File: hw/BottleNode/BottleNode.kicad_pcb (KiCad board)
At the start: 2 copper layers, 29 x 40 mm, 16 parts, among them J1 Conn_01x03_Pin, J2 Conn_01x02_Pin

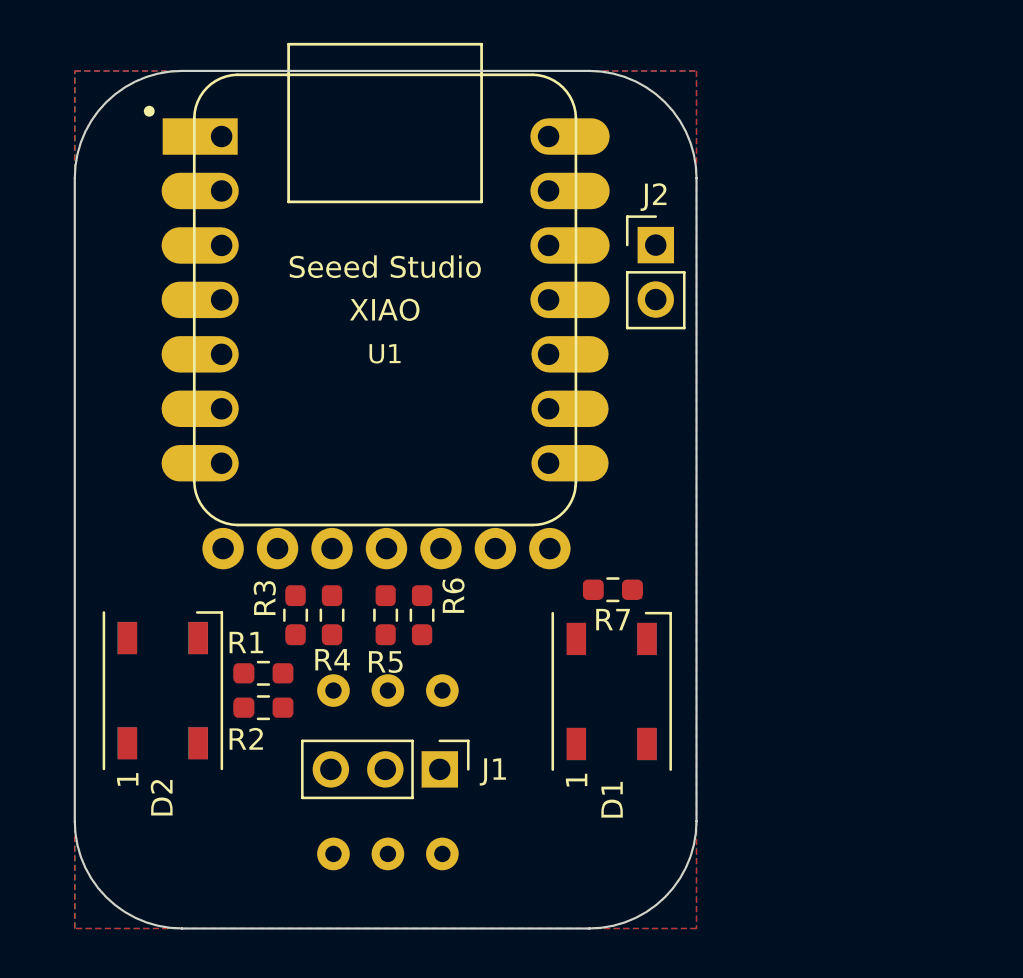
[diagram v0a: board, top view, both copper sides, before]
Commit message: rev 1.1 of schematic and PCB layout with BOM
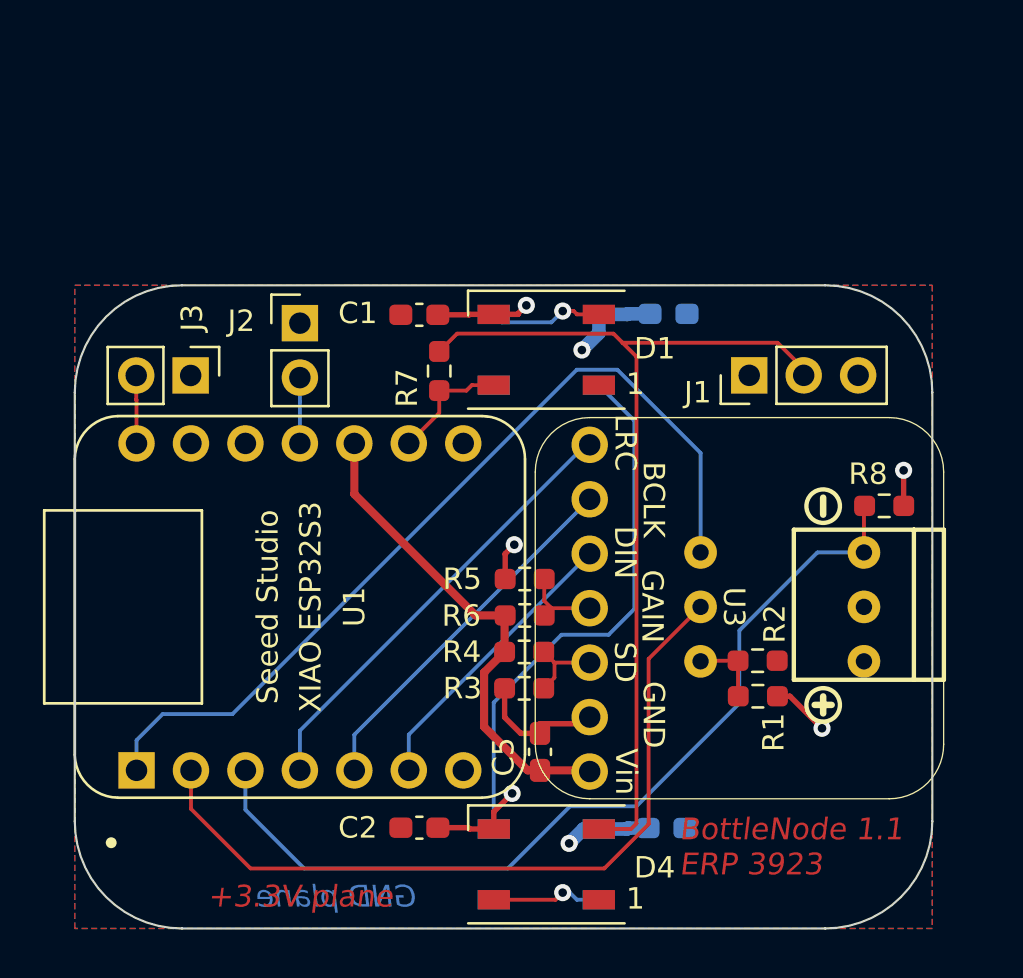
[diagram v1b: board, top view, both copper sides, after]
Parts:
- added C1: 10nF, BottleNode:C_0603_1608Metric_Pad1.08x0.95mm_HandSolder, F.Cu at (101.1, 77.4)
- added C2: 10nF, BottleNode:C_0603_1608Metric_Pad1.08x0.95mm_HandSolder, F.Cu at (101.1, 101.3)
- added C3: 10nF, BottleNode:C_0603_1608Metric_Pad1.08x0.95mm_HandSolder, B.Cu at (112.6, 101.3)
- added C4: 10nF, BottleNode:C_0603_1608Metric_Pad1.08x0.95mm_HandSolder, B.Cu at (112.7, 77.3)
- added C5: 1uF, BottleNode:C_0603_1608Metric_Pad1.08x0.95mm_HandSolder, F.Cu at (106.7, 97.8)
- added J3: Conn_01x02_Pin, BottleNode:PinHeader_1x02_P2.54mm_Vertical, F.Cu at (90.4, 80.2)
- added R8: 100k, BottleNode:R_0603_1608Metric_Pad0.98x0.95mm_HandSolder, F.Cu at (122.8, 86.3)
- D1, D3: footprint LED_SMD:LED_WS2812B_PLCC4_5.0x5.0mm_P3.2mm -> BottleNode:LED_WS2812B_PLCC4_5.0x5.0mm_P3.2mm
- D2: footprint LED_SMD:LED_WS2812B_PLCC4_5.0x5.0mm_P3.2mm -> BottleNode:LED_WS2812B_PLCC4_5.0x5.0mm_P3.2mm; moved to B.Cu
- D4: footprint LED_SMD:LED_WS2812B_PLCC4_5.0x5.0mm_P3.2mm -> BottleNode:LED_WS2812B_PLCC4_5.0x5.0mm_P3.2mm; moved to F.Cu
- J1: footprint Connector_PinHeader_2.54mm:PinHeader_1x03_P2.54mm_Vertical -> BottleNode:PinHeader_1x03_P2.54mm_Vertical
- J2: footprint Connector_PinHeader_2.54mm:PinHeader_1x02_P2.54mm_Vertical -> BottleNode:PinHeader_1x02_P2.54mm_Vertical
- R1, R2, R3, R4, R5, R6, R7: footprint Resistor_SMD:R_0603_1608Metric_Pad0.98x0.95mm_HandSolder -> BottleNode:R_0603_1608Metric_Pad0.98x0.95mm_HandSolder
- U1: footprint Seeed Studio XIAO Series Library:XIAO-Generic-Hybrid-14P-2.54-21X17.8MM -> BottleNode:XIAO-Generic-Thruhole-14P-2.54-21X17.8MM
- U2: footprint BottleNode_footprints:INMP441_breakout -> BottleNode:INMP441_breakout
- U3: footprint BottleNode_footprints:MAX98357A_adafruit_breakout -> BottleNode:MAX98357A_adafruit_breakout; moved to F.Cu
- moved D2 23.9 mm to (107.0, 79.0), turned to 180 degrees
- moved J1 23.4 mm to (116.5, 80.2), turned to 90 degrees
- moved R2 23.2 mm to (116.9, 93.5), turned to 180 degrees
- moved R1 23.1 mm to (116.9, 95.2), turned to 0 degrees
- moved U2 19.9 mm to (118.0, 91.0), turned to 90 degrees
- moved D3 19.6 mm to (107.0, 103.0), turned to 180 degrees
- moved U3 19.1 mm to (116.0, 91.0), turned to -90 degrees
- moved J2 17.0 mm to (95.5, 77.8)
- moved D1 16.2 mm to (107.0, 79.0), turned to 180 degrees
- moved U1 14.9 mm to (95.5, 91.0), turned to 90 degrees
- moved R7 13.0 mm to (102.0, 80.0), turned to -90 degrees
- moved R3 11.2 mm to (106.0, 94.8), turned to 180 degrees
- moved R4 9.12 mm to (106.0, 93.1), turned to 0 degrees
- moved D4 8.62 mm to (107.0, 103.0), turned to 180 degrees
- moved R5 6.70 mm to (106.0, 89.7), turned to 180 degrees
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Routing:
- net Net-(D4-DOUT): track 0.00 -> 42.5 mm
- net /MIC_SD: track 0.00 -> 42.1 mm
- net /MIC_SCK: track 0.00 -> 41.1 mm
- net /MIC_WS: track 0.00 -> 36.3 mm
- net Net-(D2-DOUT): track 0.00 -> 25.4 mm
- net /SPKR_POWER: track 0.00 -> 23.1 mm
- net GND: track 0.00 -> 21.3 mm, vias 0 -> 5
- net /SPKR_LRC: track 0.00 -> 20.9 mm
- net /SPKR_BCLK: track 0.00 -> 17.2 mm
- net /SPKR_DIN: track 0.00 -> 13.6 mm
- net +3.3V: track 0.00 -> 8.36 mm, vias 0 -> 2
- net /LED_DIN: track 0.00 -> 5.70 mm
- net Net-(D1-DOUT): track 0.00 -> 5.33 mm, vias 0 -> 1
- net Net-(D3-DOUT): track 0.00 -> 5.17 mm, vias 0 -> 1
- net /SPKR_GAIN: track 0.00 -> 3.76 mm
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- added copper zone on F.Cu, net +3.3V
- removed copper zone on F.Cu, net GND
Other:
- board size 29 x 40 mm -> 40 x 30 mm
- board text added: "+3.3V plane"
- board text added: "BottleNode 1.1 ERP 3923"
- board text added: "GND plane"

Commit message: final tweaks on PCB v1.1
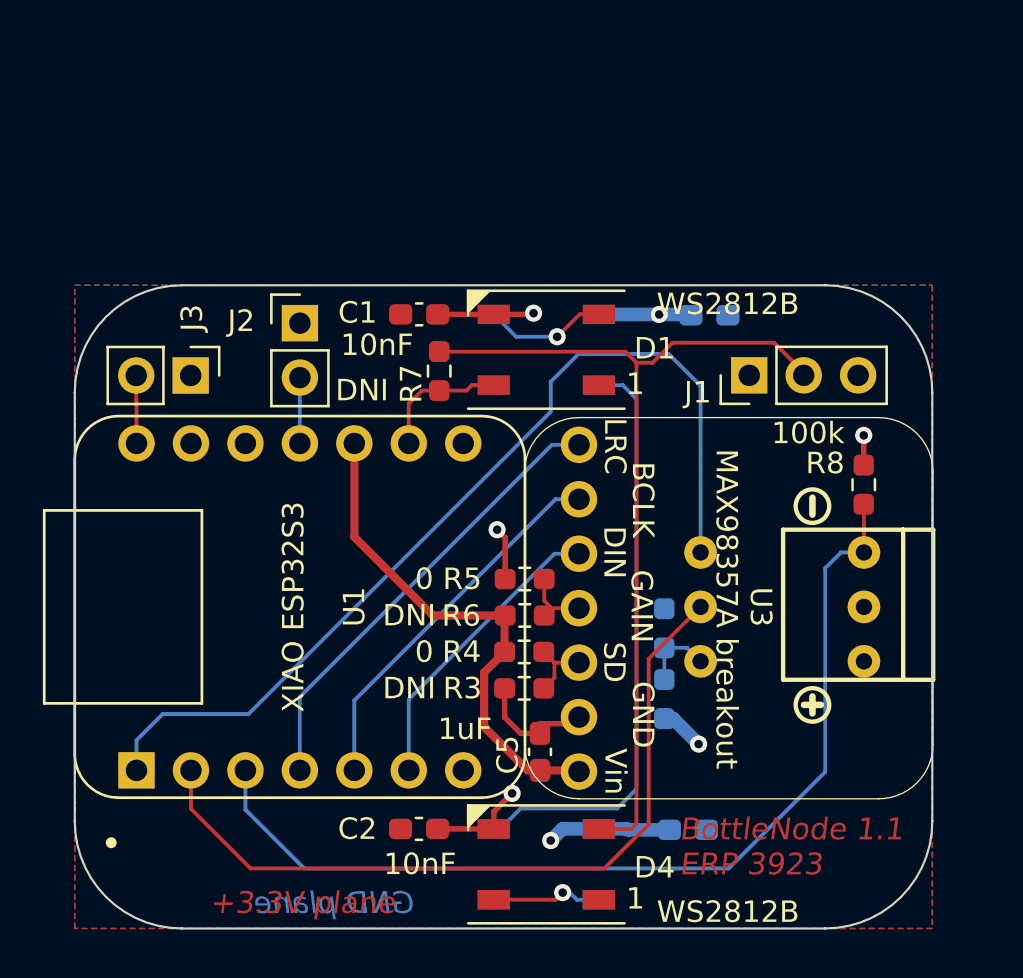
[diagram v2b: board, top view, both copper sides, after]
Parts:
- R1, R2: moved to B.Cu
- U1: value ~ -> XIAO ESP32S3
- U2: value ~ -> INMP441 breakout
- U3: value ~ -> MAX98357A breakout
- moved R1 5.39 mm to (112.5, 92.0), turned to 90 degrees
- moved R2 4.70 mm to (112.5, 95.3), turned to 90 degrees
- moved C4 1.91 mm to (114.6, 77.4)
- moved R8 1.37 mm to (121.8, 85.3), turned to -90 degrees
- moved C3 1.00 mm to (113.6, 101.4)
- moved U3 0.50 mm to (115.5, 91.0)
- moved C2 0.06 mm to (101.1, 101.4)
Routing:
- net +3.3V: track 8.36 -> 12.2 mm, vias 2 -> 3
- net /MIC_SD: track 42.1 -> 45.7 mm
- net /MIC_SCK: track 41.1 -> 44.4 mm
- net Net-(D2-DOUT): track 25.4 -> 27.6 mm
- net GND: track 21.3 -> 19.2 mm, vias 5 -> 4
- net Net-(D4-DOUT): track 42.5 -> 41.3 mm
- net /SPKR_POWER: track 23.1 -> 24.3 mm
- net /SPKR_DIN: track 13.6 -> 14.6 mm
- net /SPKR_BCLK: track 17.2 -> 18.1 mm
- net /SPKR_LRC: track 20.9 -> 21.8 mm
